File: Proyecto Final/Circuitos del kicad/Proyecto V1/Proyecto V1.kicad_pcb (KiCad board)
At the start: 2 copper layers, 107.5 x 98.6 mm, 31 parts, among them J1 12v, J2 I2C + LCD, J3 DS1307, J4 Encoder, K1 RAYEX-L90, K2 RAYEX-L90, K3 RAYEX-L90, Q1 PN2222A, Q2 PN2222A, Q3 PN2222A, SW1 SW_Push, SW2 SW_Push, SW3 SW_Push, SW4 SW_Push, U1 LM7805, U2 DS18B20, U3 ATmega328P-P, Y1 16MHz

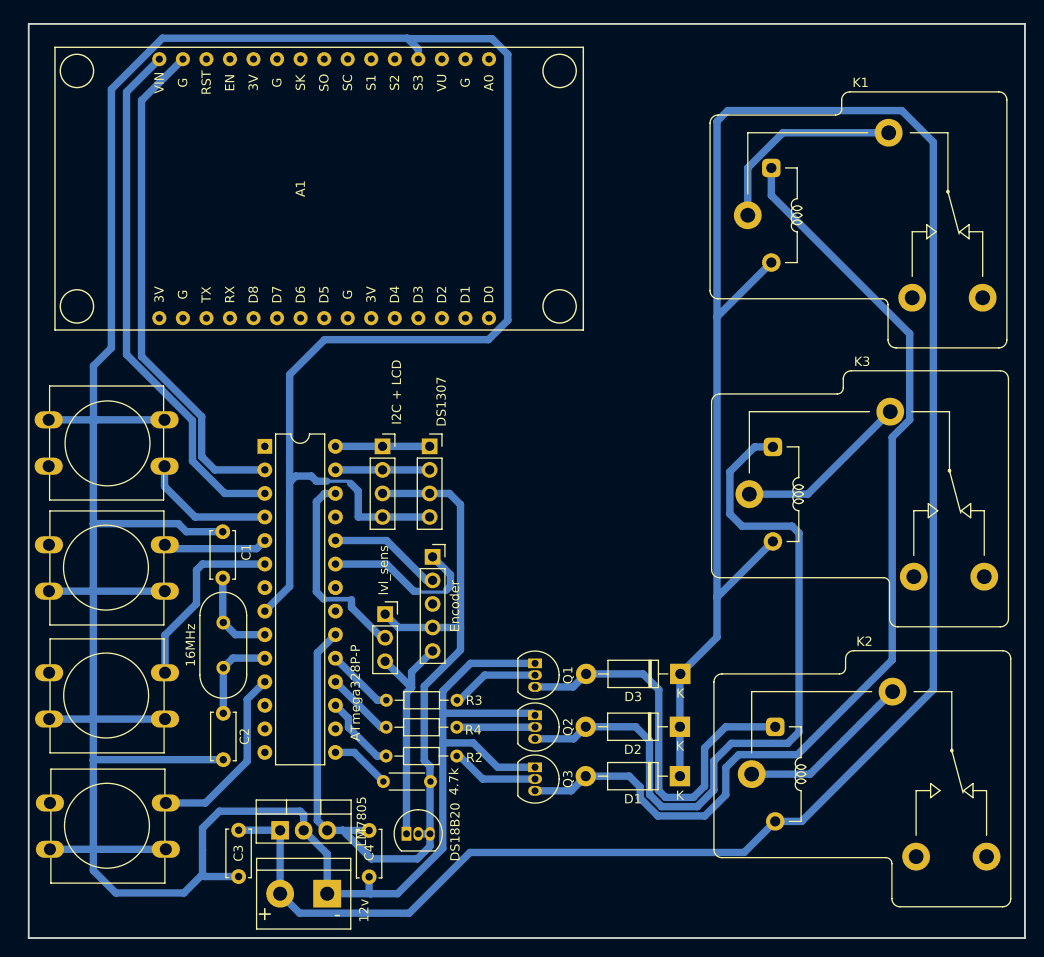
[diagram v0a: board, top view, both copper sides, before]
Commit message: cambios pene
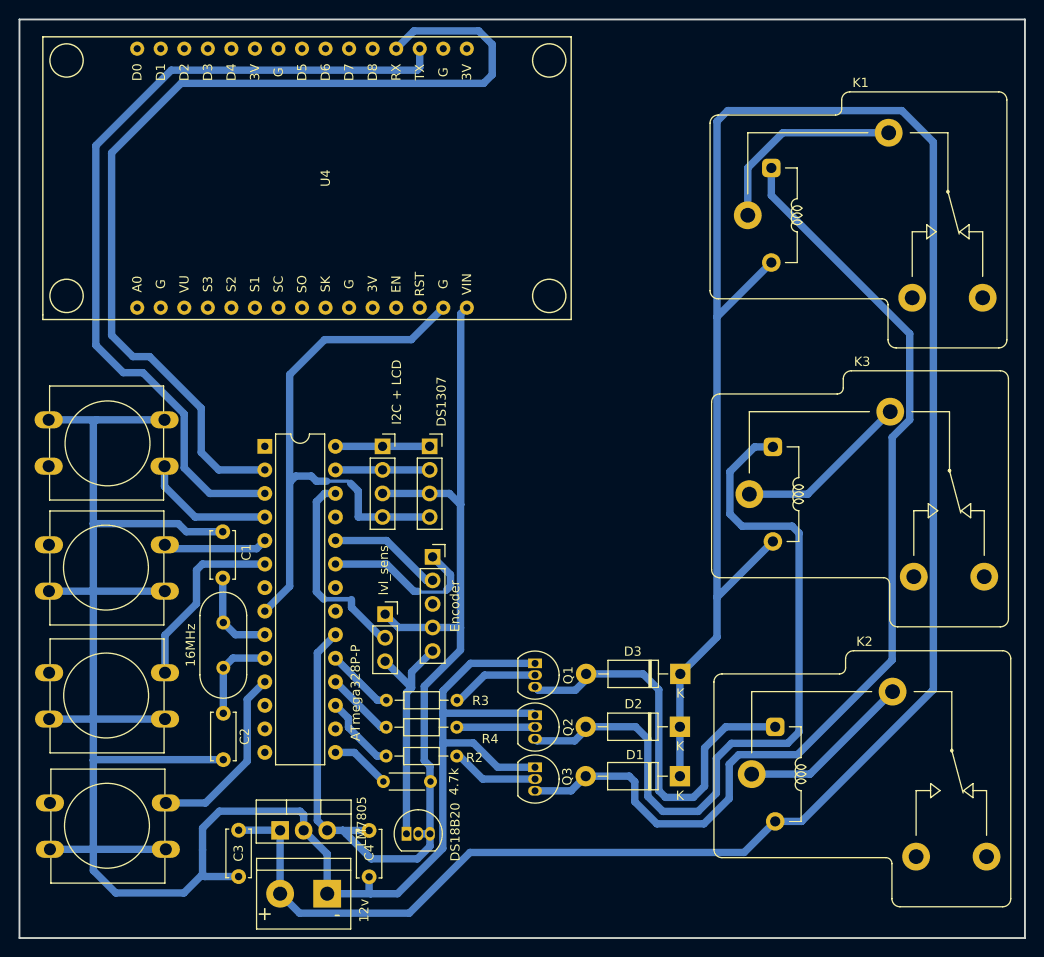
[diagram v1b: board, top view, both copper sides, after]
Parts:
- removed A1: ESP8266, ESP8266 LOLiN v3:ESP8266
- added U4: NodeMCU1.0(ESP-12E), ESP8266 LOLiN v3:ESP8266, F.Cu at (151.3, 56.2)
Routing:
- net GND: track 447.2 -> 327.1 mm
- net Net-(U3-Pad2): track 54.8 -> 104.6 mm
- net Net-(U3-Pad3): track 57.0 -> 90.3 mm
- net +5V: track 95.8 -> 117.3 mm
- net Net-(D1-Pad2): track 110.4 -> 112.1 mm
- net Net-(D2-Pad2): track 81.2 -> 82.6 mm
- net Net-(D3-Pad2): track 44.0 -> 44.6 mm
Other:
- board size 107.5 x 98.6 mm -> 108.5 x 99.1 mm
